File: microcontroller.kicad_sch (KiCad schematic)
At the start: 20 parts, among them SW1 A6S-2104-H, U6 STM32H725RGV6, Y1 ECS-2520MV-240-BN

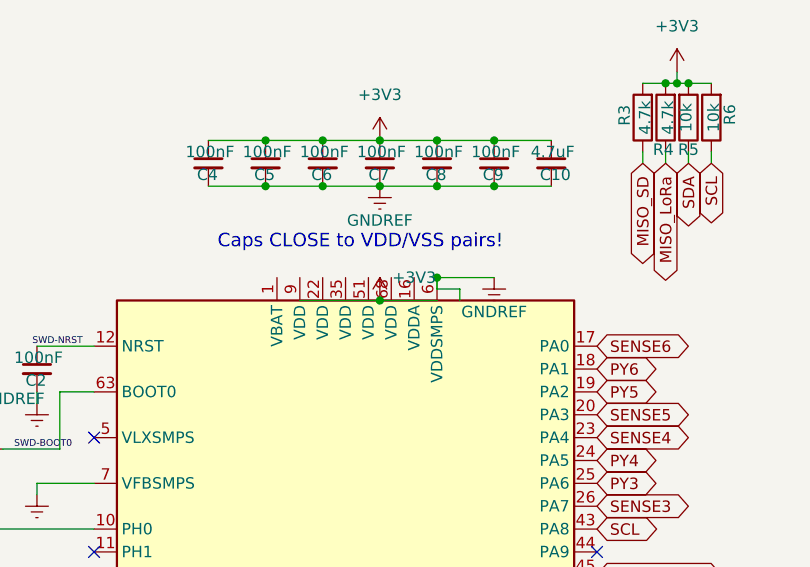
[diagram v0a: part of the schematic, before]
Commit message: Some layout tweaks
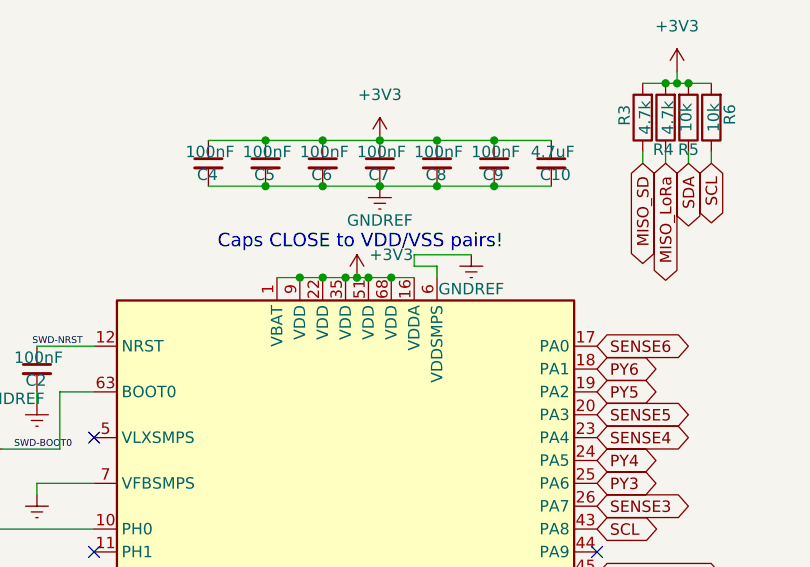
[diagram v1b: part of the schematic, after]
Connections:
- net +3V3: now also U6.1 (VBAT), U6.16 (VDDA), U6.22 (VDD), U6.35 (VDD), U6.51 (VDD), U6.68 (VDD), U6.9 (VDD)
